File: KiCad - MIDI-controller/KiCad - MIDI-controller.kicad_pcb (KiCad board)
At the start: 2 copper layers, 66 parts, among them SW1 SW_Push, SW10 SW_Push, SW11 SW_Push, SW12 SW_Push, SW13 SW_Push, SW14 SW_Push, SW15 SW_Push, SW16 SW_Push, SW17 SW_Push, SW18 SW_Push, SW19 SW_Push, SW2 SW_Push, SW20 SW_Push, SW21 RotaryEncoder_Switch, SW22 RotaryEncoder_Switch, SW23 RotaryEncoder_Switch, SW3 SW_Push, SW4 SW_Push, SW5 SW_Push, SW6 SW_Push, SW7 SW_Push, SW8 SW_Push, SW9 SW_Push, U1 ESP32-S3-WROOM-1, U2 CD74HC4067M, U3 CD74HC4067M

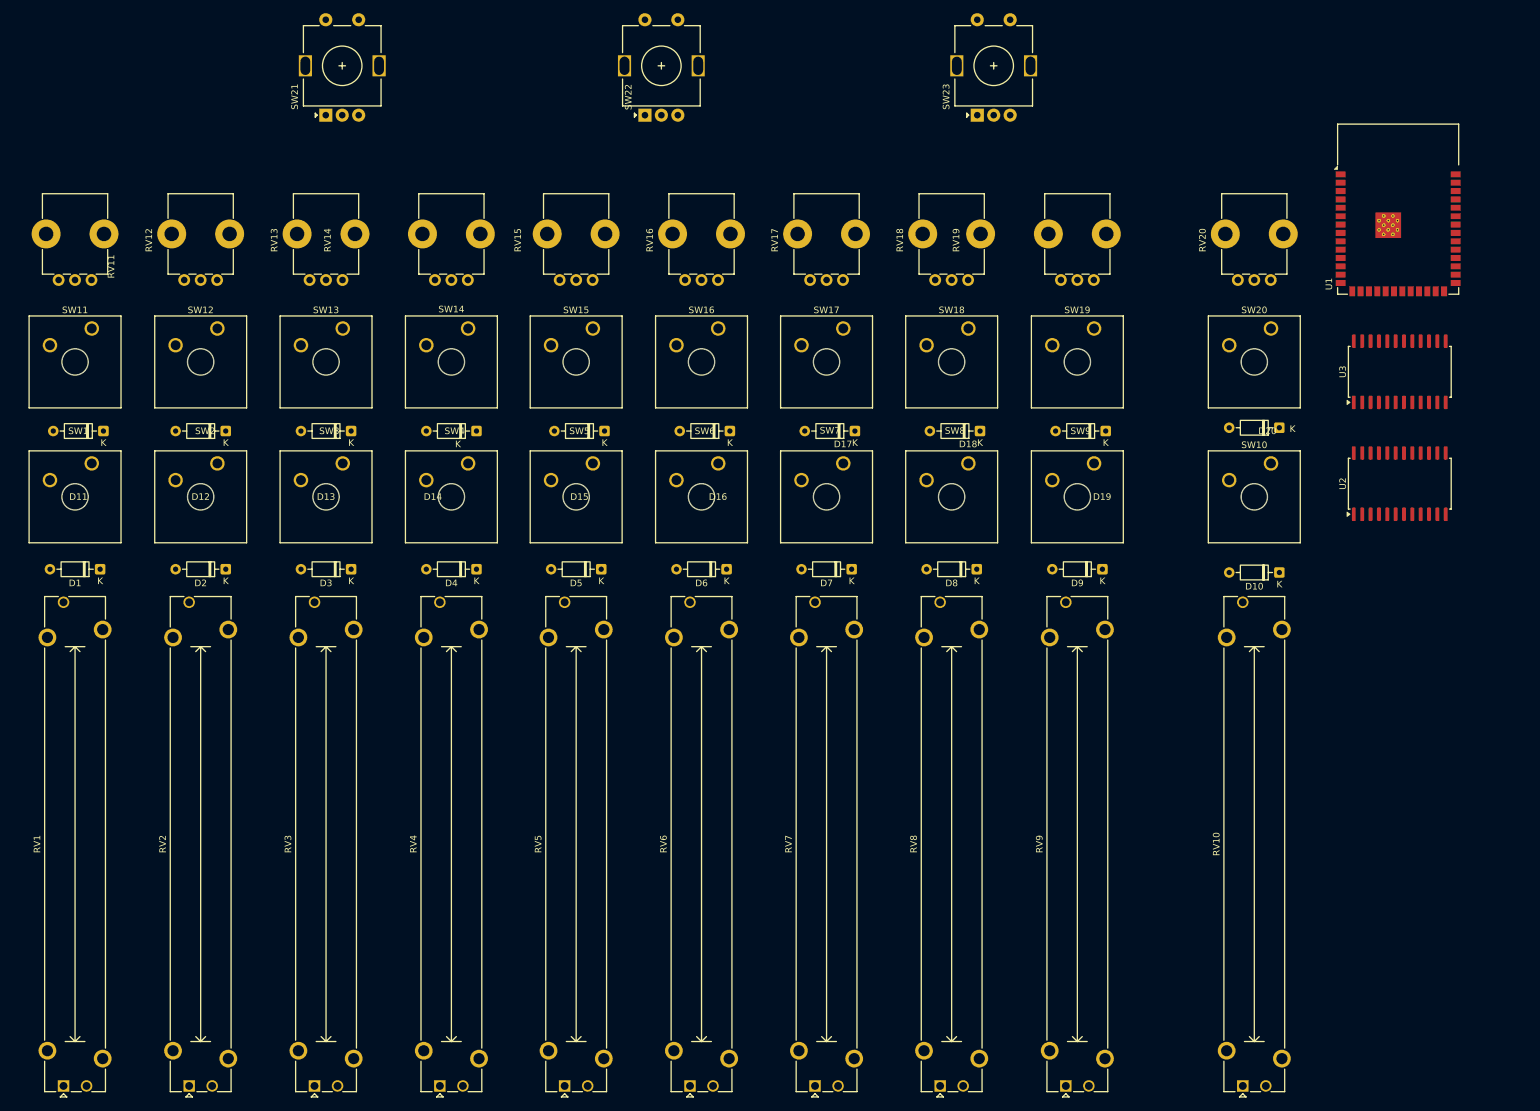
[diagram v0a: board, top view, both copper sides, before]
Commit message: Day 5
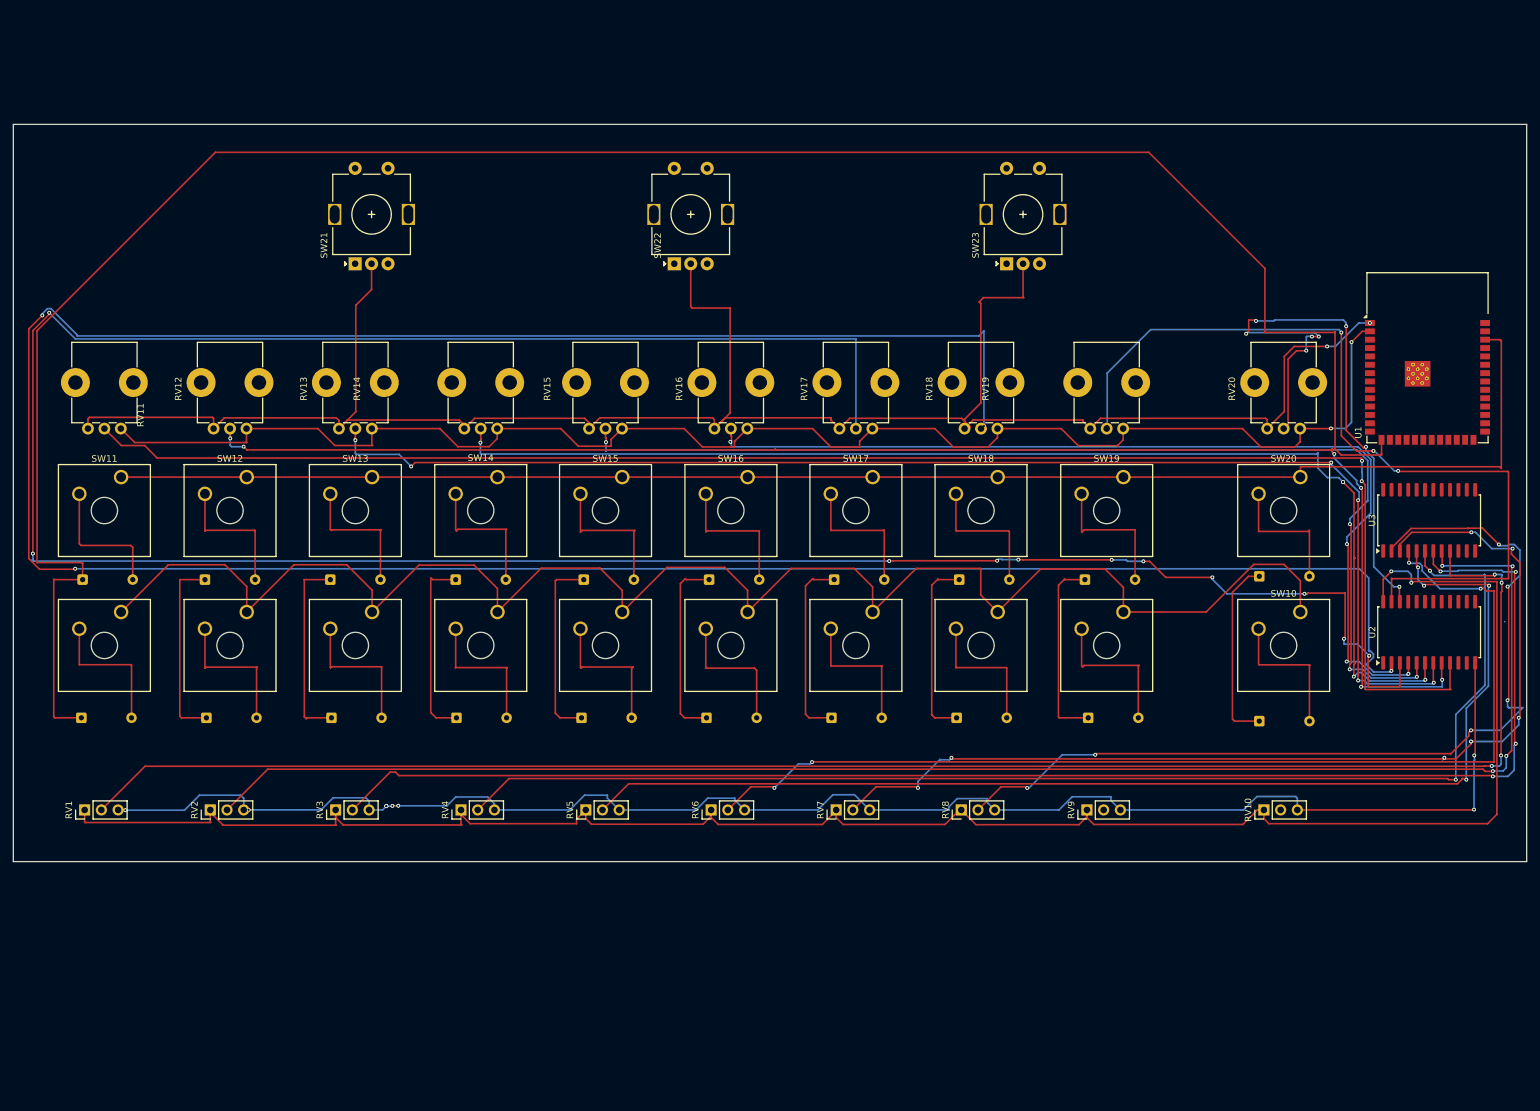
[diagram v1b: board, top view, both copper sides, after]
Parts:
- D1, D10, D11, D12, D13, D14, D15, D16, D17, D18, D19, D2, D20, D3, D4, D5, D6, D7, D8, D9: moved to B.Cu
- RV1, RV10, RV2, RV3, RV4, RV5, RV6, RV7, RV8, RV9: footprint Potentiometer_THT:Potentiometer_Bourns_PTA6043_Single_Slide -> Connector_PinHeader_2.54mm:PinHeader_1x03_P2.54mm_Vertical
- moved RV10 42.1 mm to (220.3, 139.6)
- moved RV3 42.1 mm to (79.3, 139.6)
- moved RV4 42.1 mm to (98.3, 139.6)
- moved RV6 42.1 mm to (136.3, 139.6)
- moved RV7 42.1 mm to (155.3, 139.6)
- moved RV8 42.1 mm to (174.4, 139.6)
- moved RV9 42.1 mm to (193.5, 139.6)
- moved RV1 42.1 mm to (41.1, 139.6)
- moved RV2 42.1 mm to (60.2, 139.6)
- moved RV5 42.1 mm to (117.3, 139.6)
- moved U1 23.0 mm to (245.2, 70.8)
- moved RV13 23.0 mm to (84.8, 81.6)
- moved RV14 23.0 mm to (103.8, 81.6)
- moved RV16 23.0 mm to (141.8, 81.6)
- moved RV17 23.0 mm to (160.8, 81.6)
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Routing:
- net Net-(U2-GND): track 0.00 -> 565.0 mm, vias 0 -> 10
- net Net-(U1-3V3): track 0.00 -> 533.4 mm, vias 0 -> 4
- net /POT8: track 0.00 -> 423.4 mm, vias 0 -> 4
- net /POT7: track 0.00 -> 404.1 mm, vias 0 -> 11
- net /C0l1: track 0.00 -> 327.3 mm
- net /FAD1: track 0.00 -> 256.3 mm, vias 0 -> 4
- net /ROW1: track 0.00 -> 250.2 mm
- net /POT1: track 0.00 -> 245.4 mm, vias 0 -> 2
- net /FAD2: track 0.00 -> 241.4 mm, vias 0 -> 4
- net /ROW2: track 0.00 -> 233.4 mm
- net /FAD3: track 0.00 -> 225.1 mm, vias 0 -> 4
- net /POT2: track 0.00 -> 224.7 mm, vias 0 -> 6
- net /POT3: track 0.00 -> 203.0 mm, vias 0 -> 6
- net /FAD4: track 0.00 -> 195.8 mm, vias 0 -> 2
- net /POT4: track 0.00 -> 183.2 mm, vias 0 -> 5
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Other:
- board outline added: 230 x 112 mm
